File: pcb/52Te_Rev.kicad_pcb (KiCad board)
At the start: 2 copper layers, 163.7 x 145.6 mm, 63 parts, among them J1 MJ-4PP-9, SW1 SW_PUSH, SW10 SW_PUSH, SW11 SW_PUSH, SW12 SW_PUSH, SW13 SW_PUSH, SW14 SW_PUSH, SW15 SW_PUSH, SW16 SW_PUSH, SW17 SW_PUSH, SW18 SW_PUSH, SW19 SW_PUSH, SW2 SW_PUSH, SW20 SW_PUSH, SW21 SW_PUSH, SW22 SW_PUSH, SW23 SW_PUSH, SW24 SW_PUSH, SW25 SW_PUSH, SW26 SW_PUSH, SW27 SW_PUSH, SW3 SW_PUSH, SW4 SW_PUSH, SW5 SW_PUSH, SW6 SW_PUSH, SW7 SW_PUSH, SW8 SW_PUSH, SW9 SW_PUSH, U1 ProMicro

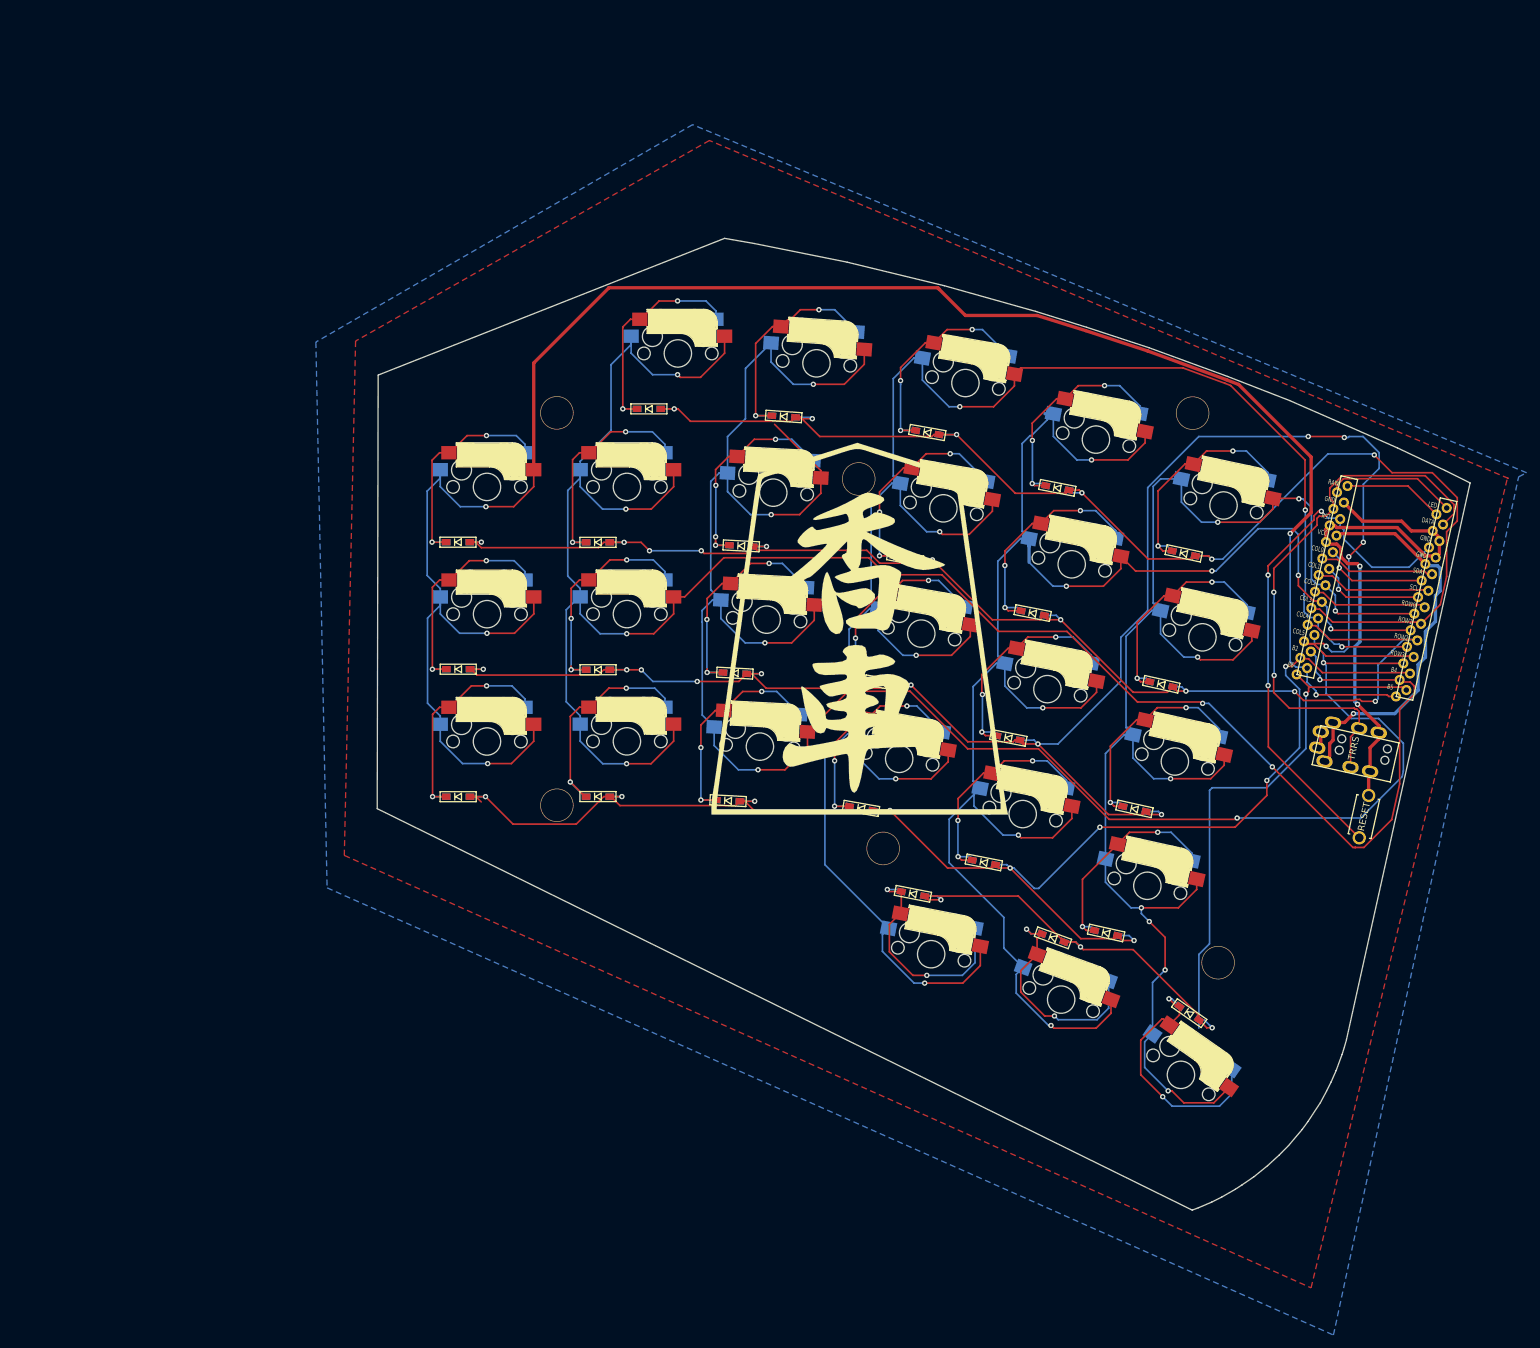
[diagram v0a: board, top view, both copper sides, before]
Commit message: redo pcb
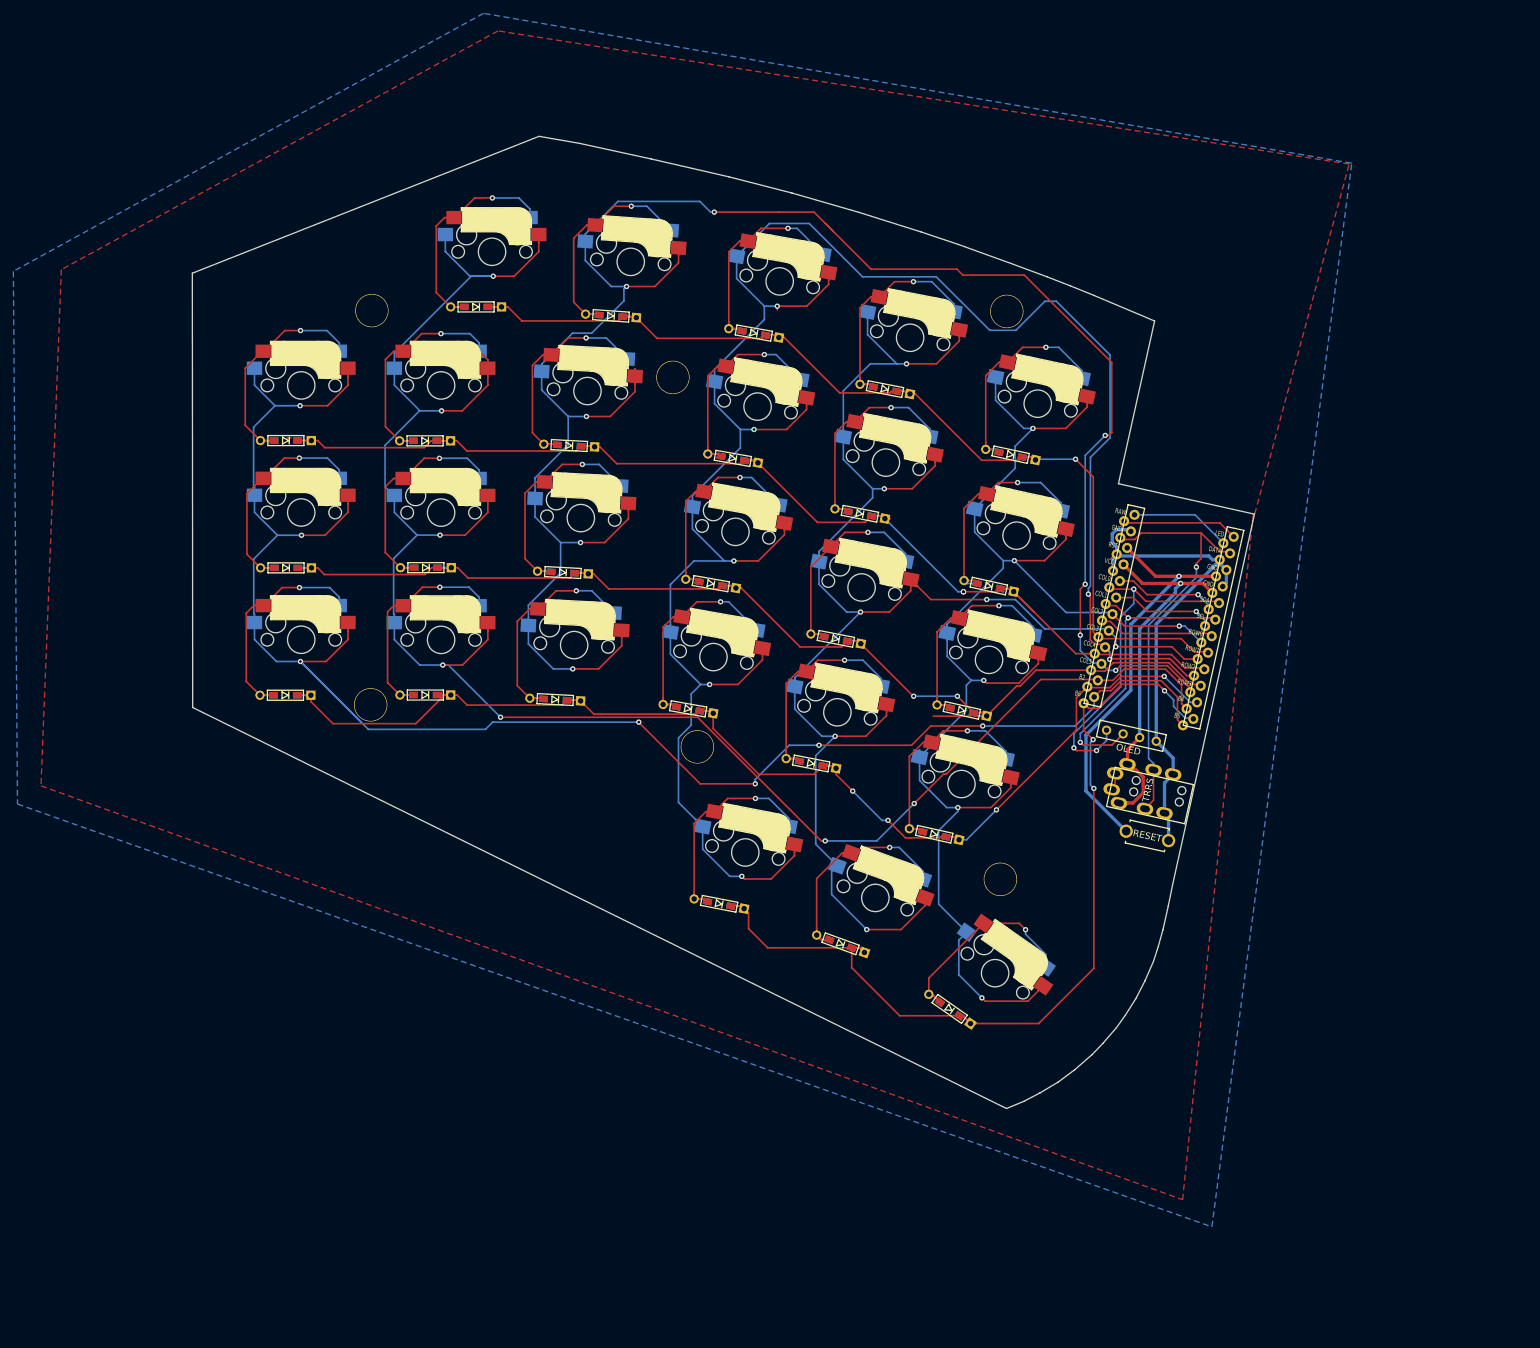
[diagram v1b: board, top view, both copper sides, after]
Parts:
- removed G***: LOGO, 52Te_Rev:kyosha
- removed G***: LOGO, 52Te_Rev:bisha
- removed the Ref** at (177.3, 172.2)
- removed the Ref** at (177.3, 113.4)
- removed the Ref** at (222.5, 123.3)
- removed the Ref** at (226.2, 178.7)
- removed the Ref** at (276.4, 195.8)
- removed the Ref** at (272.5, 113.5)
- added J2: Conn_01x04, kbd:OLED, F.Cu at (267.1, 162.6)
- added Ref**: Val**, kbd:HOLE, F.Cu at (149.6, 98.1)
- added Ref**: Val**, kbd:HOLE, F.Cu at (149.4, 157.2)
- added Ref**: Val**, kbd:HOLE, F.Cu at (198.4, 163.4)
- added Ref**: Val**, kbd:HOLE, F.Cu at (194.7, 108.1)
- added Ref**: Val**, kbd:HOLE, F.Cu at (244.7, 98.2)
- added Ref**: Val**, kbd:HOLE, F.Cu at (243.8, 183.3)
- D1, D10, D11, D12, D13, D14, D15, D16, D17, D18, D19, D2, D20, D21, D22, D23, D24, D25, D26, D3, D4, D5, D6, D7, D8, D9: footprint kbd:D3_SMD -> kbd:D3_TH_SMD
- moved D26 35.9 mm to (236.2, 202.7), turned to 145 degrees
- moved SW27 32.6 mm to (265.8, 176.8), turned to 167.5 degrees
- moved U1 32.2 mm to (268.1, 144.5)
- moved D21 31.8 mm to (219.8, 192.9), turned to 160 degrees
- moved SW16 31.7 mm to (205.5, 179.3)
- moved SW25 31.7 mm to (237.9, 169.0)
- moved SW17 31.7 mm to (230.2, 102.2)
- moved SW22 31.7 mm to (249.3, 112.0)
- moved SW23 31.7 mm to (246.2, 131.8)
- moved SW13 31.7 mm to (207.4, 112.5)
- moved SW14 31.7 mm to (204.1, 131.2)
- moved SW18 31.7 mm to (226.6, 120.9)
- moved SW2 31.7 mm to (139.0, 128.3)
- moved SW26 31.7 mm to (243.0, 197.3)
- moved SW19 31.7 mm to (223.0, 139.6)
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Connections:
- D1 pad 1: Net-(D1-Pad1) -> row1
- D1 pad 2: row1 -> Net-(D1-Pad2)
- D10 pad 1: Net-(D10-Pad1) -> row2
- D10 pad 2: row2 -> Net-(D10-Pad2)
- D11 pad 1: Net-(D11-Pad1) -> row3
- D11 pad 2: row3 -> Net-(D11-Pad2)
- D12 pad 1: Net-(D12-Pad1) -> row0
- D12 pad 2: row0 -> Net-(D12-Pad2)
- D13 pad 1: Net-(D13-Pad1) -> row1
- D13 pad 2: row1 -> Net-(D13-Pad2)
- D14 pad 1: Net-(D14-Pad1) -> row2
- D14 pad 2: row2 -> Net-(D14-Pad2)
- D15 pad 1: Net-(D15-Pad1) -> row3
- D15 pad 2: row3 -> Net-(D15-Pad2)
- D16 pad 1: Net-(D16-Pad1) -> row4
- D16 pad 2: row4 -> Net-(D16-Pad2)
- D17 pad 1: Net-(D17-Pad1) -> row0
- D17 pad 2: row0 -> Net-(D17-Pad2)
- D18 pad 1: Net-(D18-Pad1) -> row1
- D18 pad 2: row1 -> Net-(D18-Pad2)
- D19 pad 1: Net-(D19-Pad1) -> row2
- D19 pad 2: row2 -> Net-(D19-Pad2)
- D2 pad 1: Net-(D2-Pad1) -> row2
- D2 pad 2: row2 -> Net-(D2-Pad2)
- D20 pad 1: Net-(D20-Pad1) -> row3
- D20 pad 2: row3 -> Net-(D20-Pad2)
- D21 pad 1: Net-(D21-Pad1) -> row4
- D21 pad 2: row4 -> Net-(D21-Pad2)
- D22 pad 1: Net-(D22-Pad1) -> row0
- D22 pad 2: row0 -> Net-(D22-Pad2)
- D23 pad 1: Net-(D23-Pad1) -> row1
- D23 pad 2: row1 -> Net-(D23-Pad2)
- D24 pad 1: Net-(D24-Pad1) -> row2
- D24 pad 2: row2 -> Net-(D24-Pad2)
- D25 pad 1: Net-(D25-Pad1) -> row3
- D25 pad 2: row3 -> Net-(D25-Pad2)
- D26 pad 1: Net-(D26-Pad1) -> row4
- D26 pad 2: row4 -> Net-(D26-Pad2)
- D3 pad 1: Net-(D3-Pad1) -> row3
- D3 pad 2: row3 -> Net-(D3-Pad2)
- D4 pad 1: Net-(D4-Pad1) -> row0
- D4 pad 2: row0 -> Net-(D4-Pad2)
- D5 pad 1: Net-(D5-Pad1) -> row1
- D5 pad 2: row1 -> Net-(D5-Pad2)
- D6 pad 1: Net-(D6-Pad1) -> row2
- D6 pad 2: row2 -> Net-(D6-Pad2)
- D7 pad 1: Net-(D7-Pad1) -> row3
- D7 pad 2: row3 -> Net-(D7-Pad2)
- D8 pad 1: Net-(D8-Pad1) -> row0
- D8 pad 2: row0 -> Net-(D8-Pad2)
- D9 pad 1: Net-(D9-Pad1) -> row1
- D9 pad 2: row1 -> Net-(D9-Pad2)
- SW1 pad 2: Net-(D1-Pad1) -> Net-(D1-Pad2)
- SW10 pad 2: Net-(D10-Pad1) -> Net-(D10-Pad2)
- SW11 pad 2: Net-(D11-Pad1) -> Net-(D11-Pad2)
- SW12 pad 2: Net-(D12-Pad1) -> Net-(D12-Pad2)
- SW13 pad 2: Net-(D13-Pad1) -> Net-(D13-Pad2)
- SW14 pad 2: Net-(D14-Pad1) -> Net-(D14-Pad2)
- SW15 pad 2: Net-(D15-Pad1) -> Net-(D15-Pad2)
- SW16 pad 2: Net-(D16-Pad1) -> Net-(D16-Pad2)
- SW17 pad 2: Net-(D17-Pad1) -> Net-(D17-Pad2)
- SW18 pad 2: Net-(D18-Pad1) -> Net-(D18-Pad2)
- SW19 pad 2: Net-(D19-Pad1) -> Net-(D19-Pad2)
- SW2 pad 2: Net-(D2-Pad1) -> Net-(D2-Pad2)
- SW20 pad 2: Net-(D20-Pad1) -> Net-(D20-Pad2)
- SW21 pad 2: Net-(D21-Pad1) -> Net-(D21-Pad2)
- SW22 pad 2: Net-(D22-Pad1) -> Net-(D22-Pad2)
- SW23 pad 2: Net-(D23-Pad1) -> Net-(D23-Pad2)
- SW24 pad 2: Net-(D24-Pad1) -> Net-(D24-Pad2)
- SW25 pad 2: Net-(D25-Pad1) -> Net-(D25-Pad2)
- SW26 pad 2: Net-(D26-Pad1) -> Net-(D26-Pad2)
- SW3 pad 2: Net-(D3-Pad1) -> Net-(D3-Pad2)
- SW4 pad 2: Net-(D4-Pad1) -> Net-(D4-Pad2)
- SW5 pad 2: Net-(D5-Pad1) -> Net-(D5-Pad2)
- SW6 pad 2: Net-(D6-Pad1) -> Net-(D6-Pad2)
- SW7 pad 2: Net-(D7-Pad1) -> Net-(D7-Pad2)
- SW8 pad 2: Net-(D8-Pad1) -> Net-(D8-Pad2)
- SW9 pad 2: Net-(D9-Pad1) -> Net-(D9-Pad2)
- U1 pad 5: Net-(U1-Pad5) -> SDA
- U1 pad 6: Net-(U1-Pad6) -> SCL
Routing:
- net row2: track 277.8 -> 171.7 mm, vias 13 -> 2
- net SDA: track 0.00 -> 52.1 mm, vias 0 -> 3
- net SCL: track 0.00 -> 46.5 mm, vias 0 -> 2
- net col0: track 303.1 -> 260.8 mm, vias 5 -> 7
- net col1: track 322.2 -> 280.4 mm
- net row3: track 221.4 -> 181.3 mm, vias 9 -> 4
- net Net-(D26-Pad1): track 38.8 -> 0.00 mm, vias 2 -> 0
- net col4: track 269.4 -> 231.2 mm, vias 8 -> 7
- net Net-(D18-Pad1): track 36.3 -> 0.00 mm, vias 3 -> 0
- net row0: track 192.3 -> 156.4 mm, vias 6 -> 1
- net Net-(D6-Pad1): track 35.1 -> 0.00 mm, vias 3 -> 0
- net Net-(D10-Pad1): track 35.0 -> 0.00 mm, vias 3 -> 0
- net Net-(D6-Pad2): track 0.00 -> 34.9 mm, vias 0 -> 1
- net Net-(D21-Pad1): track 34.9 -> 0.00 mm, vias 2 -> 0
- net Net-(D4-Pad2): track 0.00 -> 34.8 mm, vias 0 -> 1
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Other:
- board size 163.7 x 145.6 mm -> 159.1 x 145.6 mm
- board text removed: "52Te Reversible v1.0 PCB by @SA_EndlessGame"
